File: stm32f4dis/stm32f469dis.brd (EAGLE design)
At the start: 0 parts

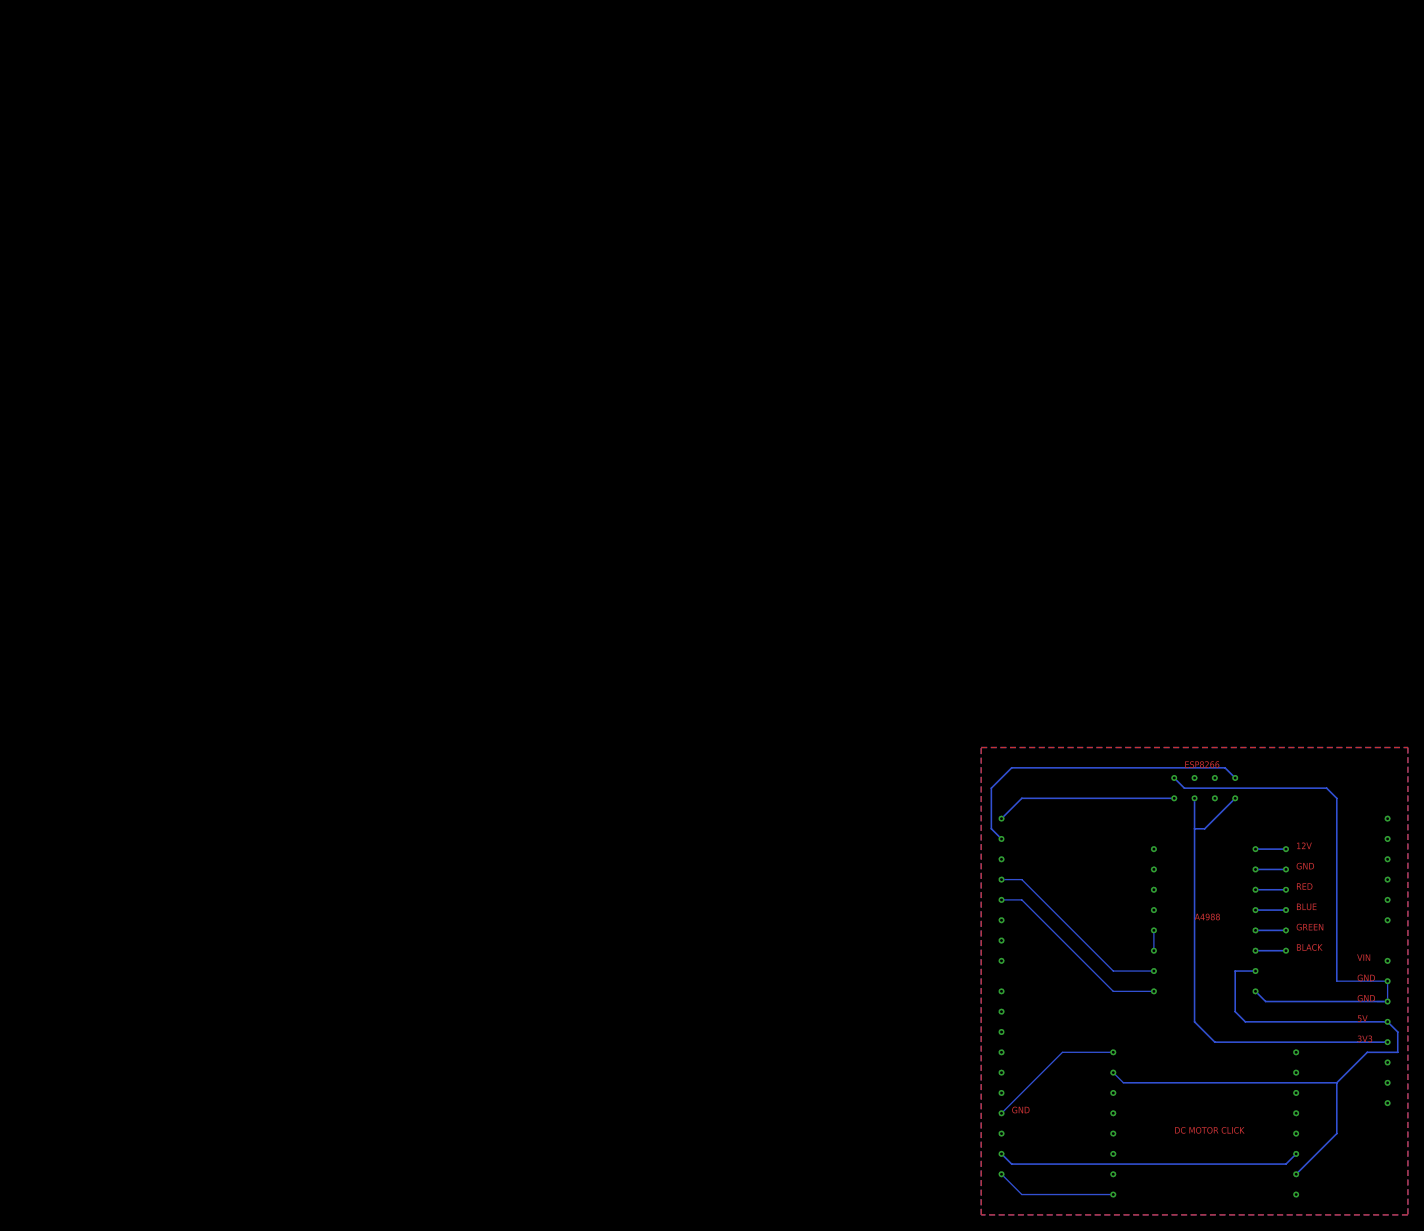
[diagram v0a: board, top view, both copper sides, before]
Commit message: eagle v2
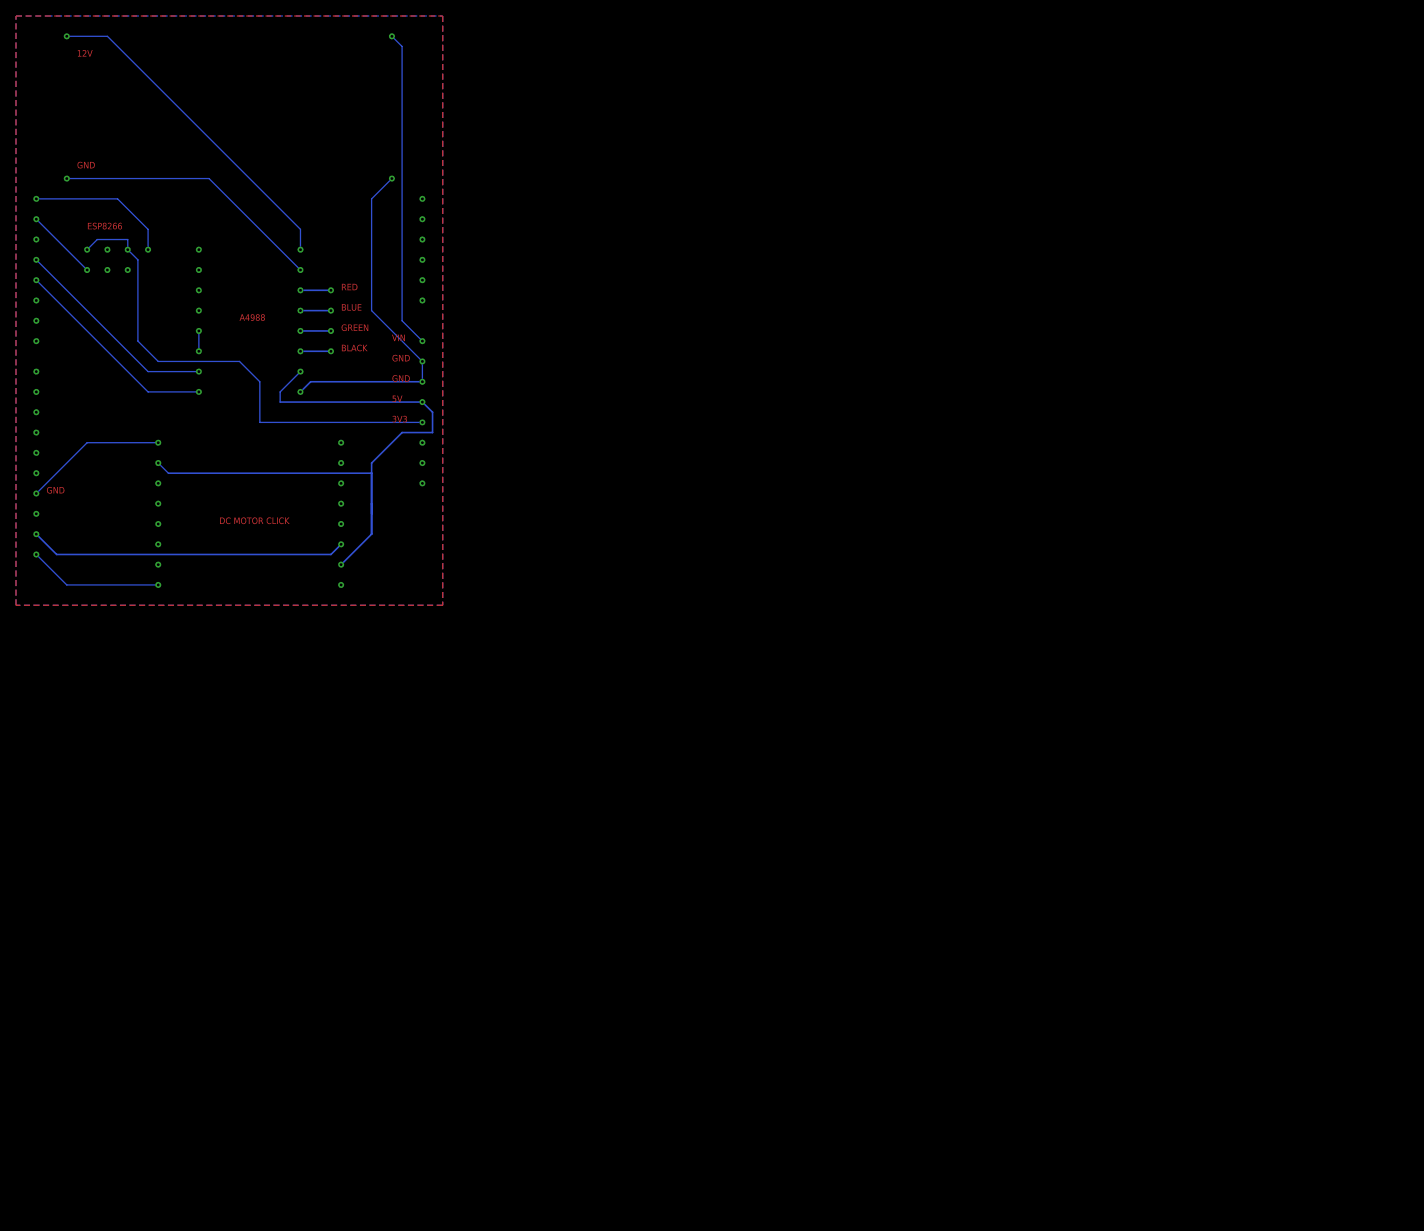
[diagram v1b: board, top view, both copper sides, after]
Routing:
- net GND: track 0.00 -> 62.7 mm, vias 0 -> 6
- net S$26: track 53.1 -> 0.00 mm, vias 3 -> 0
- net S$17: track 0.00 -> 39.7 mm, vias 0 -> 1
- net S$72: track 38.9 -> 0.00 mm, vias 2 -> 0
- net S$41: track 3.81 -> 41.7 mm, vias 1 -> 2
- net S$42: track 3.81 -> 33.9 mm, vias 1 -> 2
- net S$65: track 18.3 -> 0.00 mm, vias 1 -> 0
- net S$49: track 17.1 -> 0.00 mm, vias 1 -> 0
- net S$47: track 27.2 -> 17.8 mm, vias 1 -> 0
- net S$27: track 0.00 -> 8.98 mm, vias 0 -> 2
- net S$63: track 55.5 -> 63.9 mm
- net S$68: track 0.00 -> 4.86 mm, vias 0 -> 1
- net S$2: track 22.6 -> 18.1 mm
- net S$4: track 23.8 -> 26.1 mm
- net S$5: track 23.8 -> 26.1 mm
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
